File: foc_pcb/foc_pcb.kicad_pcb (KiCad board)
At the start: 2 copper layers, 66 parts, among them IC1 AS5600-ASOT, J1 USB_C_Receptacle_USB2.0, J10 Conn_02x03_Top_Bottom, J11 Conn_01x03, J2 Conn_01x03, J3 Conn_01x03, J4 Conn_01x04, J5 XT60PW-M, J6 XT60PW-M, J7 Conn_01x02, J8 Conn_01x02, J9 Conn_01x02, SW1 SW_Push, U1 DRV8313PWPR, U2 ATMEGA328P-AU, U3 BSS138-7-F, U4 BSS138-7-F, U5 CH340C, Y1 ABM3-16MHZ

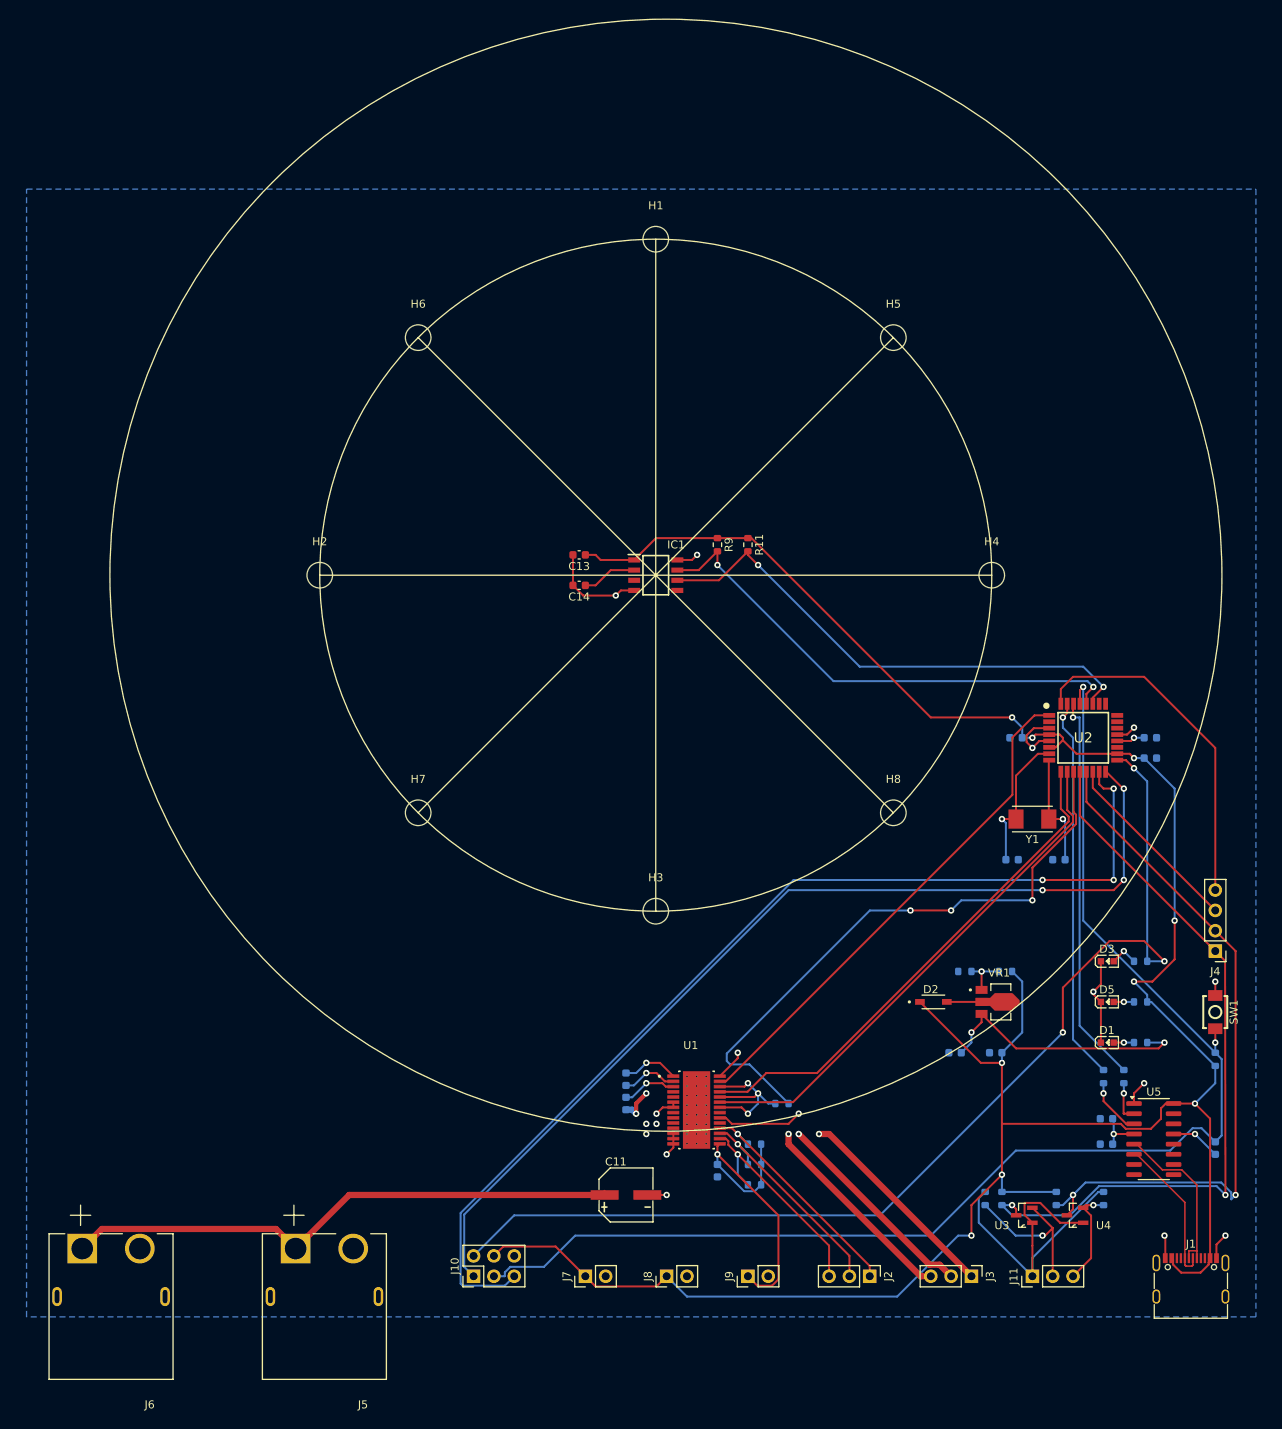
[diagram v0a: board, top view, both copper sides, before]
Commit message: before switch usb
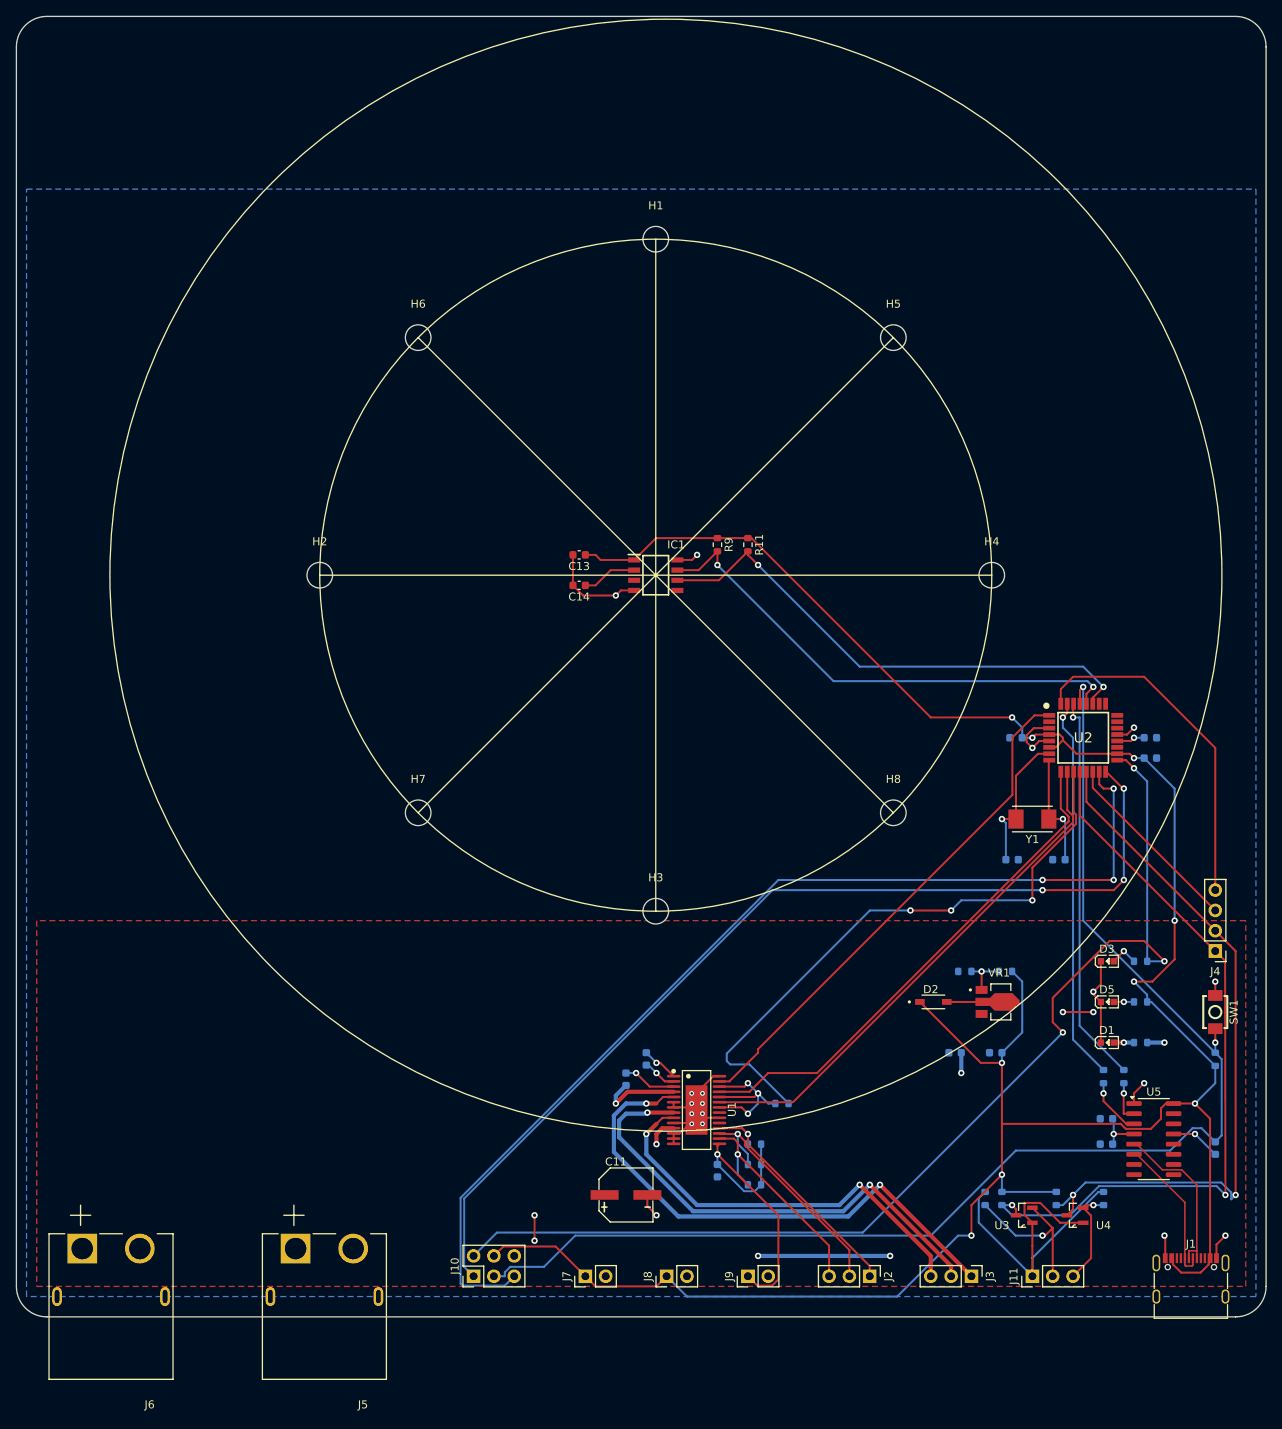
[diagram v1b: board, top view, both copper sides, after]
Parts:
- U1: footprint DRV8313PWPR:SOP65P640X120-29N -> DRV8313PWPR:HTSSOP-28_L9.8-W4.5-P0.65-LS6.6-BL-EP
- moved C2 3.59 mm to (293.4, 270.0)
- moved C3 3.03 mm to (290.8, 272.6)
- turned U1 to -90 degrees
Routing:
- net VCC: track 108.2 -> 35.5 mm, vias 4 -> 6
- net /out1: track 26.4 -> 67.4 mm
- net /out2: track 26.4 -> 61.3 mm
- net /out3: track 25.9 -> 52.3 mm
- net GND: track 70.4 -> 76.5 mm, vias 14 -> 22
- net Net-(U1-CPH): track 6.99 -> 4.26 mm
- net Net-(U1-CPL): track 7.14 -> 4.63 mm
- net /nSlp: track 28.2 -> 30.2 mm
- net /miso: track 122.6 -> 123.8 mm
- net /mosi: track 130.1 -> 131.2 mm
- net /sck: track 136.6 -> 137.6 mm
- net /nRes: track 27.6 -> 28.3 mm
- added copper zone on F.Cu, net VCC
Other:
- board outline added: 156.2 x 162.6 mm
- rule pad_to_mask_clearance: 0.038 -> 0
